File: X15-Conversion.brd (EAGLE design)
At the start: 50.8 x 62.9 mm, 27 parts, among them U1 LINEAR,AZ1117CR-3.3TRG1DIODES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

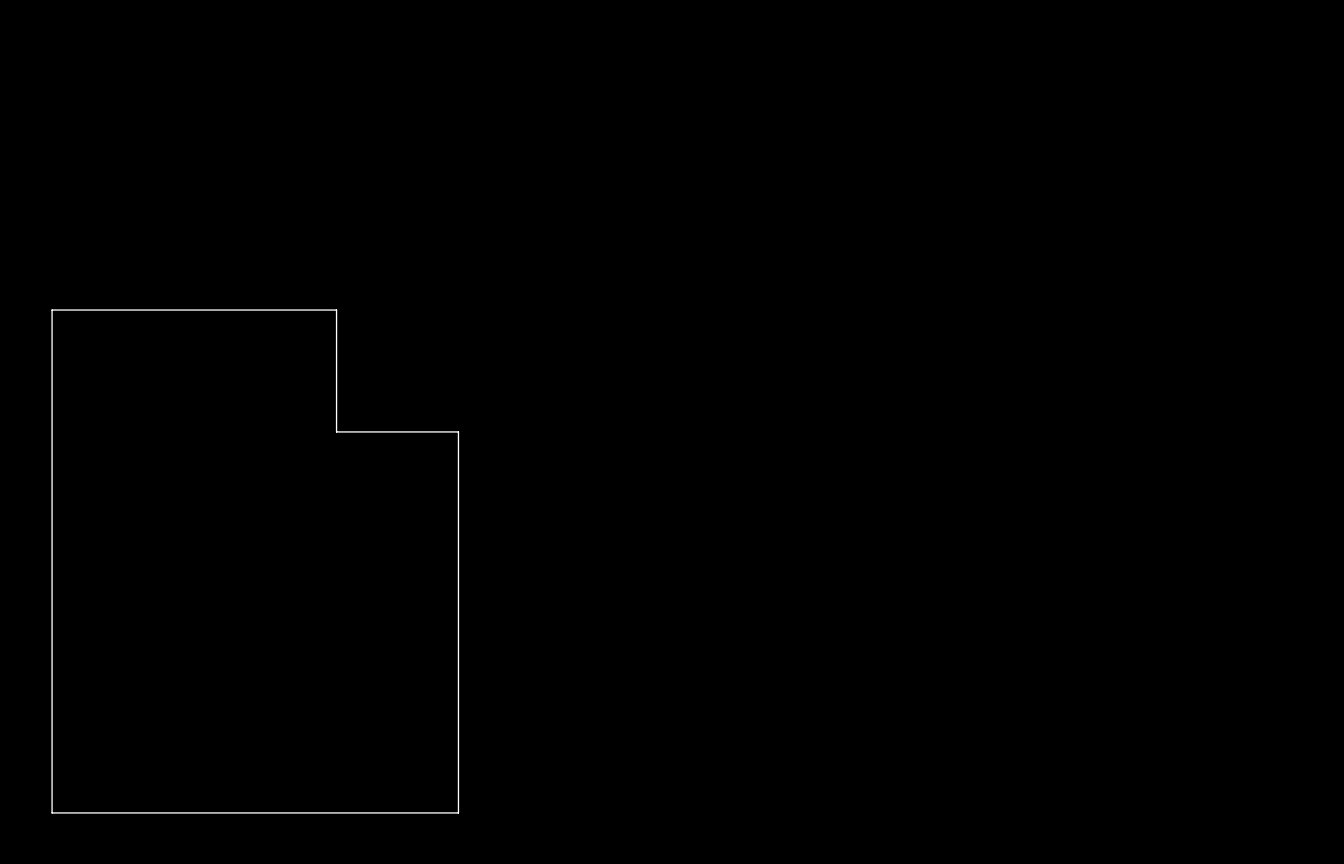
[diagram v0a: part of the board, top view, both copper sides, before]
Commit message: Revert "Merge branch 'master' of https://github.com/purduerov/X15-Conversion"
This reverts commit 41817e178b7c3d64232767e30bfff53a28a489f7, reversing
changes made to 9f5667108a341ebdd134b7c2334aa0d8aa0ab67e.
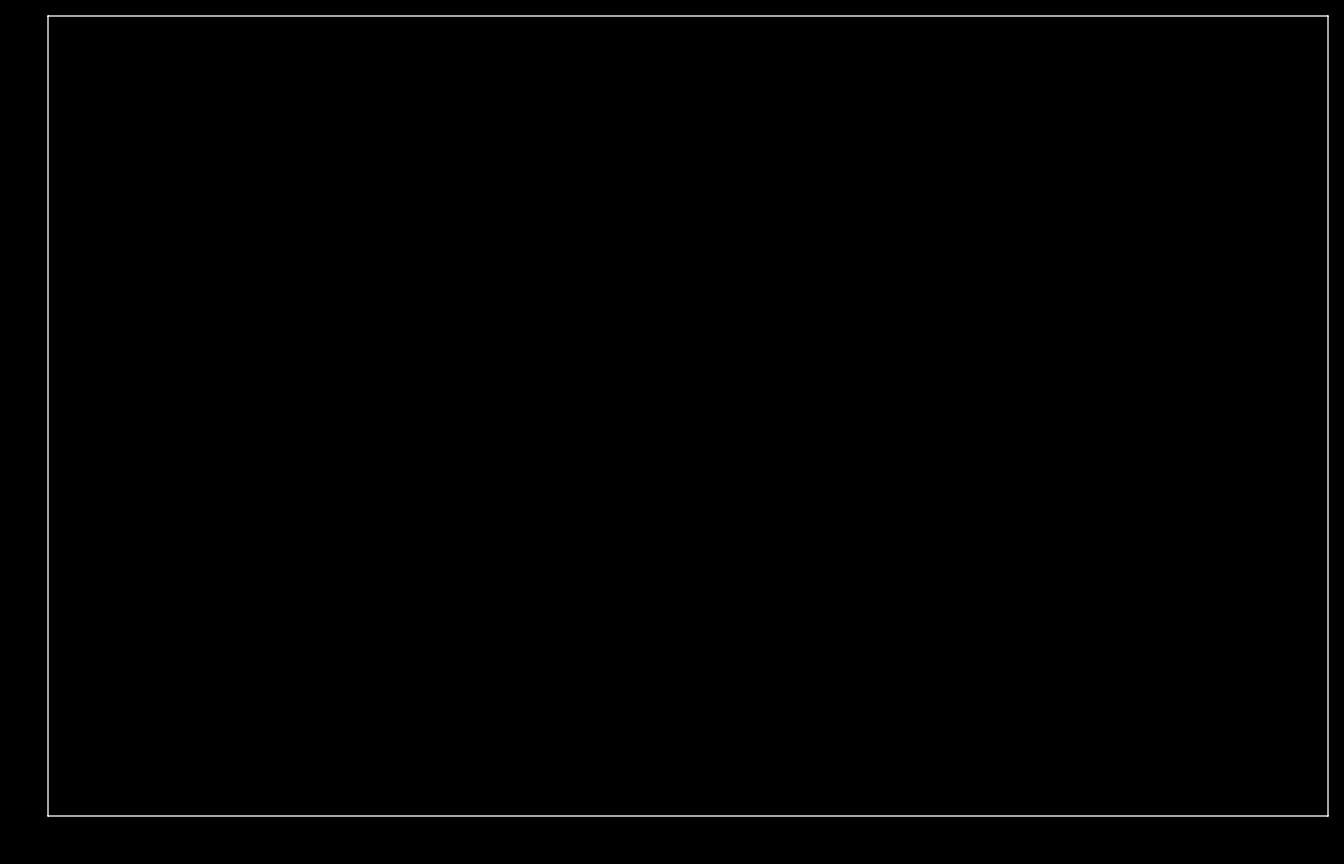
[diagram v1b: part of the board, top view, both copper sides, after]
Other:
- board size 50.8 x 62.9 mm -> 160 x 100 mm
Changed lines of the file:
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@@
 <board>
 <plain>
-<wire x1="0.508" y1="0.381" x2="51.308" y2="0.381" width="0" layer="20"/>
-<wire x1="51.308" y1="0.381" x2="51.308" y2="48.006" width="0" layer="20"/>
-<wire x1="36.068" y1="63.246" x2="0.508" y2="63.246" width="0" layer="20"/>
-<wire x1="0.508" y1="63.246" x2="0.508" y2="0.381" width="0" layer="20"/>
-<wire x1="36.068" y1="63.246" x2="36.068" y2="48.006" width="0" layer="20"/>
-<wire x1="36.068" y1="48.006" x2="51.308" y2="48.006" width="0" layer="20"/>
+<wire x1="0" y1="0" x2="160" y2="0" width="0" layer="20"/>
+<wire x1="160" y1="0" x2="160" y2="100" width="0" layer="20"/>
+<wire x1="160" y1="100" x2="0" y2="100" width="0" layer="20"/>
+<wire x1="0" y1="100" x2="0" y2="0" width="0" layer="20"/>
 </plain>
 <attributes>
